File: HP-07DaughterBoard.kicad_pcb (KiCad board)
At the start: 2 copper layers, 104.1 x 73.7 mm, 18 parts, among them J1 Barrel_Jack, J2 Firing Speed, J3 Oscillation Speed, J4 Topspin, J5 Backspin, J6 Conn_02x20_Odd_Even, Q1 FMMT493TA, Q2 FMMT493TA, Q3 FMMT493TA, Q4 FMMT493TA

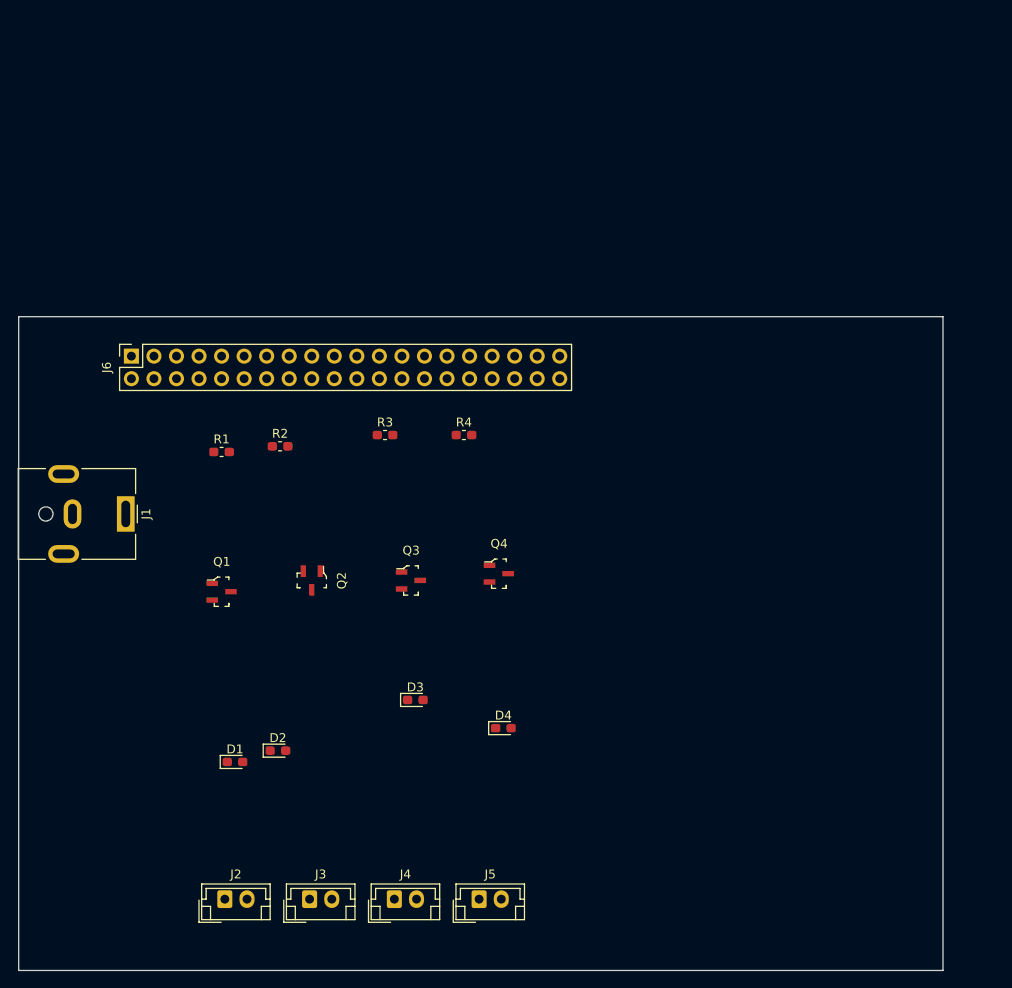
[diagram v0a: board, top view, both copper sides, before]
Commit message: Update
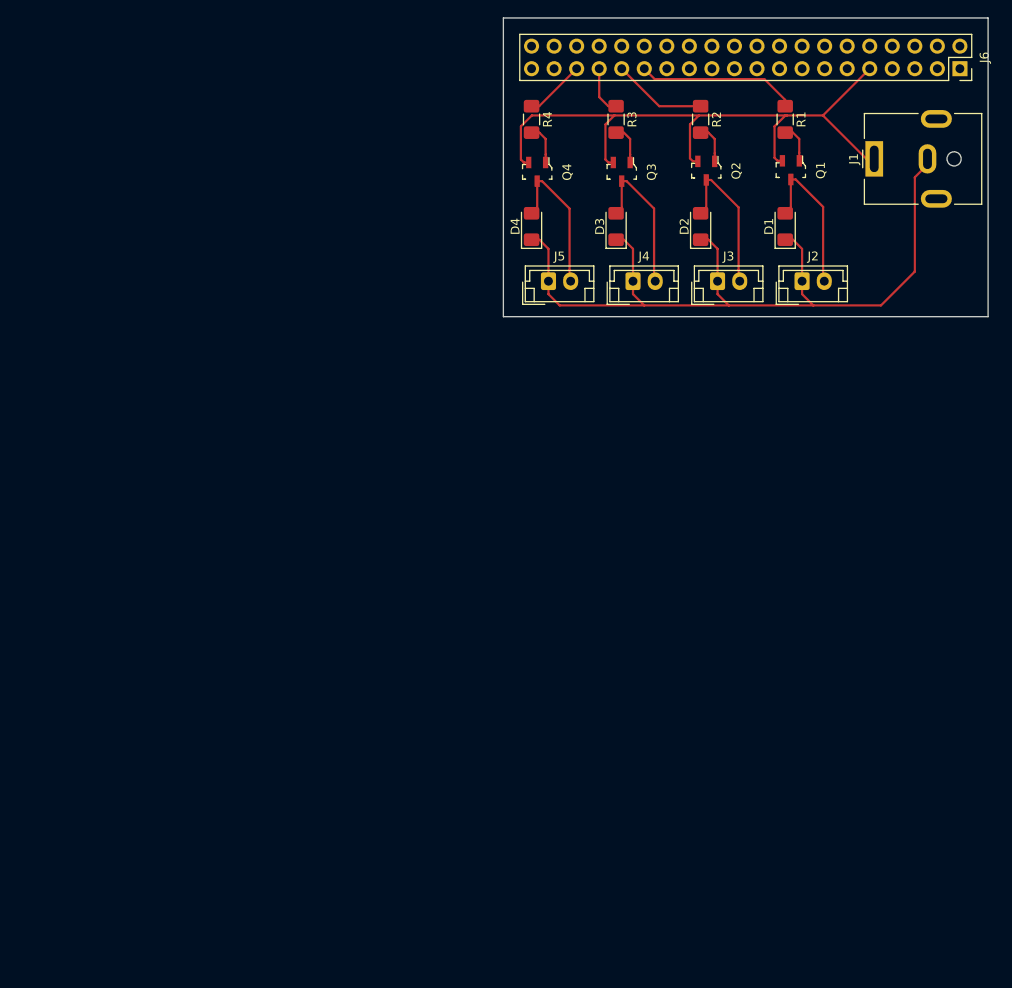
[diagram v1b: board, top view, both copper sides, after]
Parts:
- D1, D2, D3, D4: footprint Diode_SMD:D_0603_1608Metric_Pad1.05x0.95mm_HandSolder -> Diode_SMD:D_1206_3216Metric_Pad1.42x1.75mm_HandSolder
- R1, R2, R3, R4: footprint Resistor_SMD:R_0603_1608Metric_Pad1.05x0.95mm_HandSolder -> Resistor_SMD:R_1206_3216Metric_Pad1.42x1.75mm_HandSolder
- moved J6 98.8 mm to (258.4, 25.4), turned to 270 degrees
- moved J2 95.3 mm to (240.7, 49.3)
- moved J1 93.3 mm to (248.8, 35.6), turned to 90 degrees
- moved D1 86.5 mm to (238.8, 43.2), turned to 90 degrees
- moved J3 83.4 mm to (231.1, 49.3)
- moved Q1 79.8 mm to (239.4, 36.8), turned to 270 degrees
- moved D2 75.9 mm to (229.2, 43.2), turned to 90 degrees
- moved J4 74.6 mm to (221.6, 49.3)
- moved R1 73.7 mm to (238.8, 31.1), turned to 270 degrees
- moved J5 70.1 mm to (212.1, 49.3)
- moved Q2 64.1 mm to (229.9, 36.9)
- moved R2 60.0 mm to (229.2, 31.1), turned to 270 degrees
- moved D3 57.9 mm to (219.7, 43.2), turned to 90 degrees
- moved D4 56.6 mm to (210.2, 43.2), turned to 90 degrees
- moved Q3 51.8 mm to (220.3, 37.0), turned to 270 degrees
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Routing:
- net Net-(D1-Pad1): track 0.00 -> 91.8 mm
- net Net-(J1-Pad1): track 0.00 -> 74.4 mm
- net Net-(J6-Pad29): track 0.00 -> 18.0 mm
- net Net-(D1-Pad2): track 0.00 -> 17.4 mm
- net Net-(D2-Pad2): track 0.00 -> 17.3 mm
- net Net-(D4-Pad2): track 0.00 -> 17.0 mm
- net Net-(D3-Pad2): track 0.00 -> 17.0 mm
- net Net-(J6-Pad31): track 0.00 -> 10.6 mm
- net Net-(J6-Pad35): track 0.00 -> 6.83 mm
- net Net-(J6-Pad33): track 0.00 -> 5.53 mm
- net Net-(Q4-Pad1): track 0.00 -> 4.54 mm
- net Net-(Q3-Pad1): track 0.00 -> 4.54 mm
- net Net-(Q2-Pad1): track 0.00 -> 4.40 mm
- net Net-(Q1-Pad1): track 0.00 -> 4.35 mm
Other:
- board size 104.1 x 73.7 mm -> 54.6 x 33.7 mm
